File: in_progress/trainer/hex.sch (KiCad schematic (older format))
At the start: 28 parts

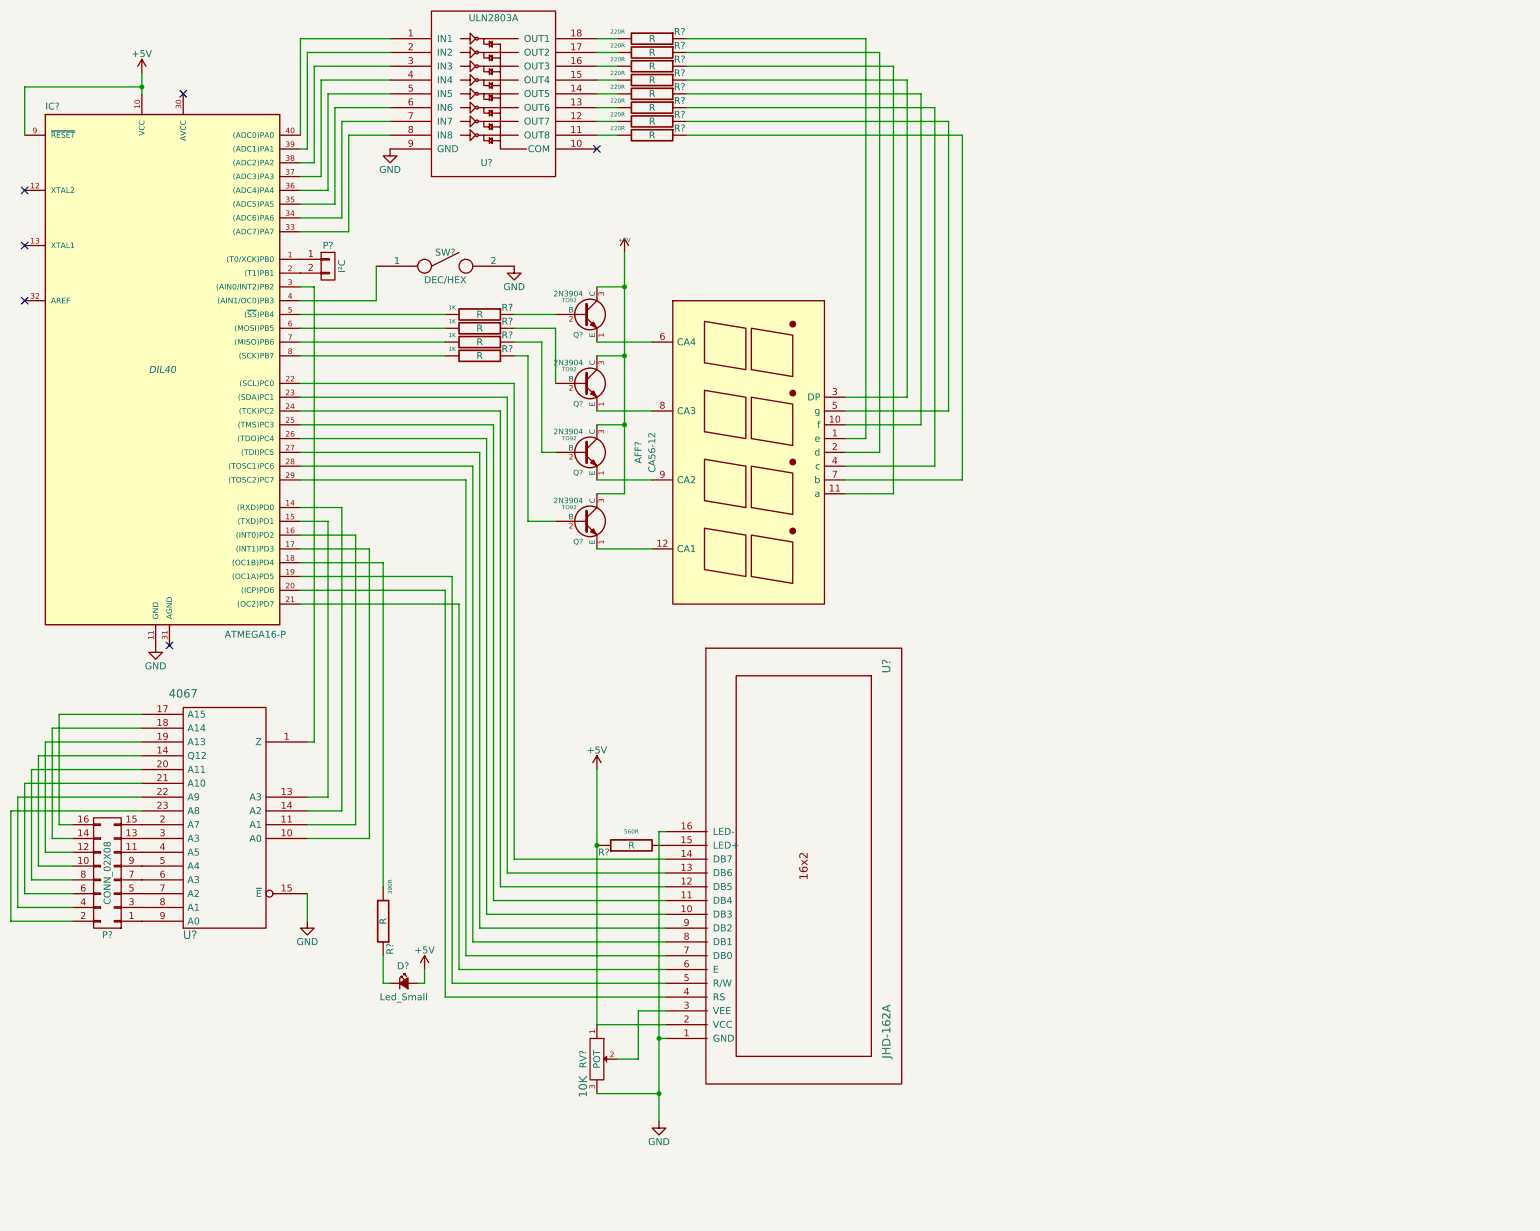
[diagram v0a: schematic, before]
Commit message: .
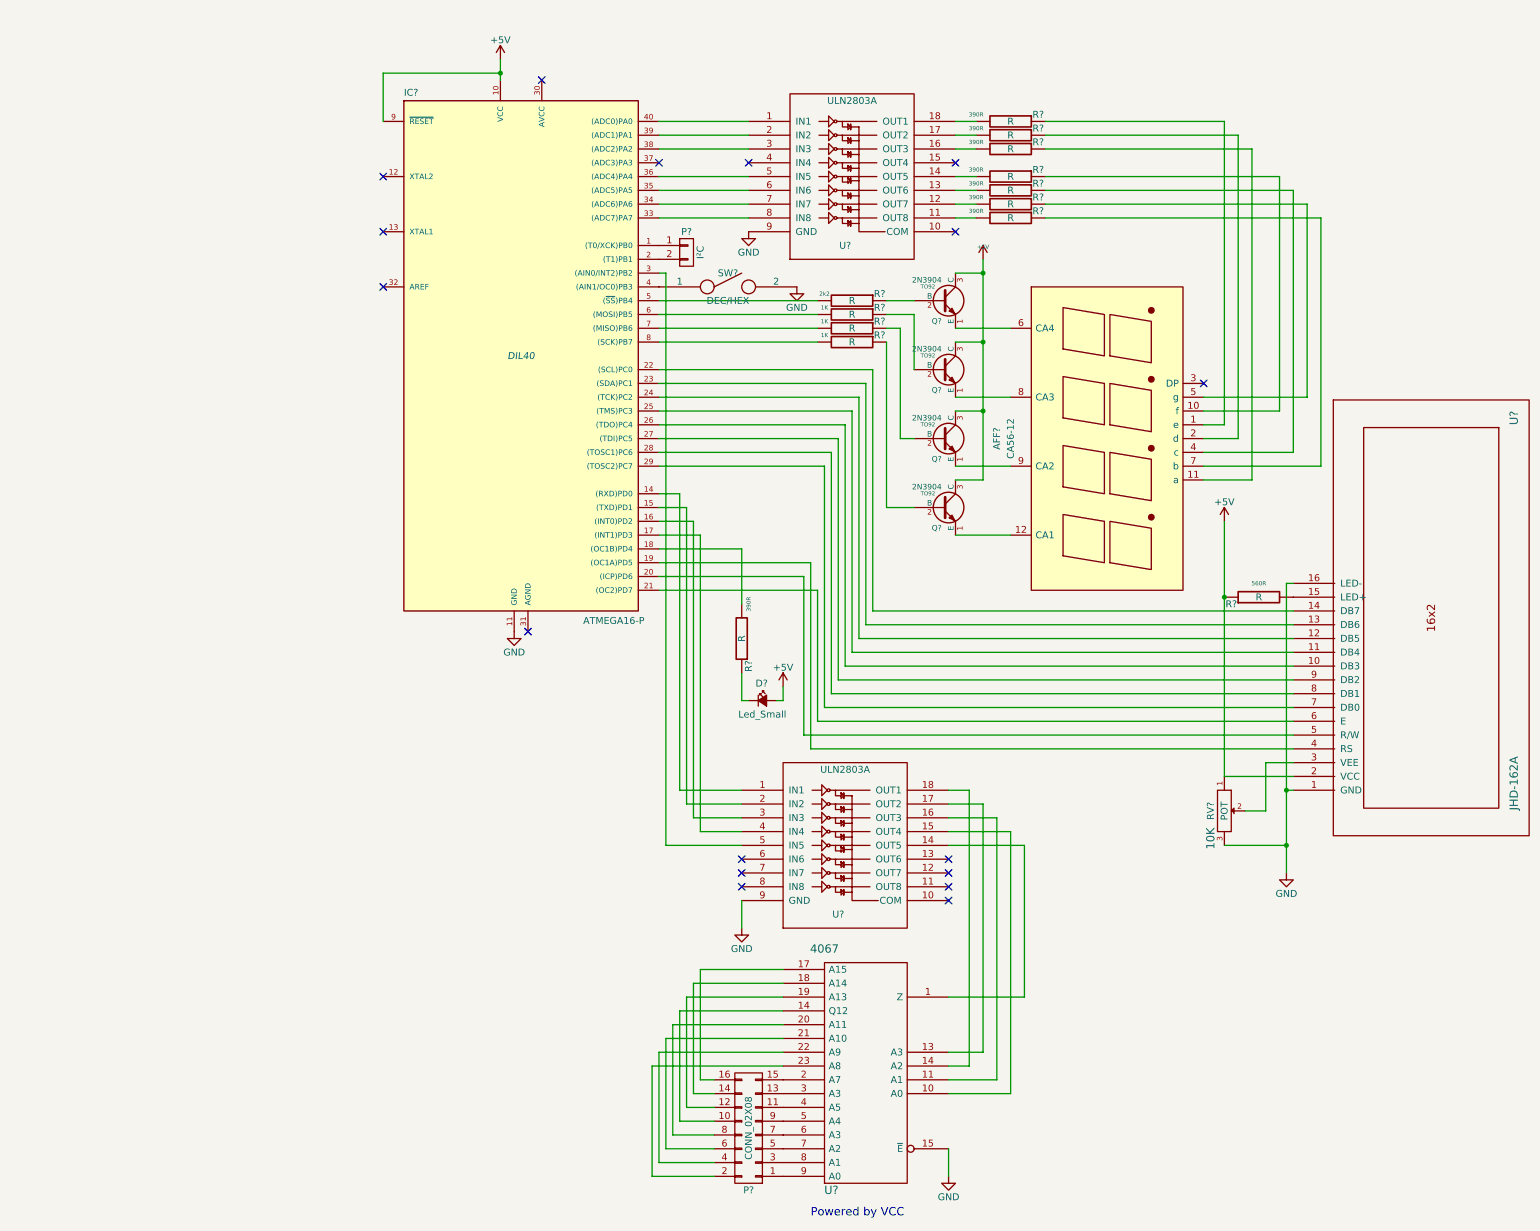
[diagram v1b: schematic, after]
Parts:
- removed R?: R, 220R, symbol R-RESCUE-trainer
- added U?: ULN2803A, symbol ULN2803A
- R? (x7): footprint 220R -> 390R
- R?: footprint 1K -> 2k2
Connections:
- net GND: now also U?.9 (GND)
- net at U?.1 (Z): now also U?.14 (OUT5); no longer IC?.3 ((AIN0/INT2)PB2)
- net at U?.10 (A0): now also U?.15 (OUT4); no longer IC?.17 ((INT1)PD3)
- net at U?.11 (A1): now also U?.16 (OUT3); no longer IC?.16 ((INT0)PD2)
- net at U?.13 (A3): now also U?.17 (OUT2); no longer IC?.15 ((TXD)PD1)
- net at U?.14 (Q12): now also U?.18 (OUT1); no longer IC?.14 ((RXD)PD0)
- net at U?.4 (IN4): no longer IC?.37 ((ADC3)PA3)
- net at IC?.19 ((OC1A)PD5): now also U?.4 (RS); no longer U?.5 (R/W)
- net at IC?.20 ((ICP)PD6): now also U?.5 (R/W); no longer U?.4 (RS)
- new net: IC?.14 ((RXD)PD0), U?.1 (IN1)
- new net: IC?.15 ((TXD)PD1), U?.2 (IN2)
- new net: IC?.16 ((INT0)PD2), U?.3 (IN3)
- new net: IC?.17 ((INT1)PD3), U?.4 (IN4)
- new net: IC?.3 ((AIN0/INT2)PB2), U?.5 (IN5)
- no-connect marks 6 -> 17
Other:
- note added: "Powered by VCC"
- moved on the sheet: AFF?, D?, IC?, P?, Q?, R?, RV?, SW?, U?
